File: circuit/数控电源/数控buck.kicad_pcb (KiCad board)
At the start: 2 copper layers, 50 x 50 mm, 80 parts, among them J1 Conn_01x06_MountingPin, J2 Conn_01x02, J5 Conn_01x02, Q1 BSC070N10NS3G, Q2 BSC070N10NS3G, SW1 SW_Push, U1 STM32F334R8Tx, U2 LM5164DDA, U4 LM5109MA, U5 INA240A1PW, U6 TLV9062, U8 LM2675M-5, Y1 Crystal_GND24

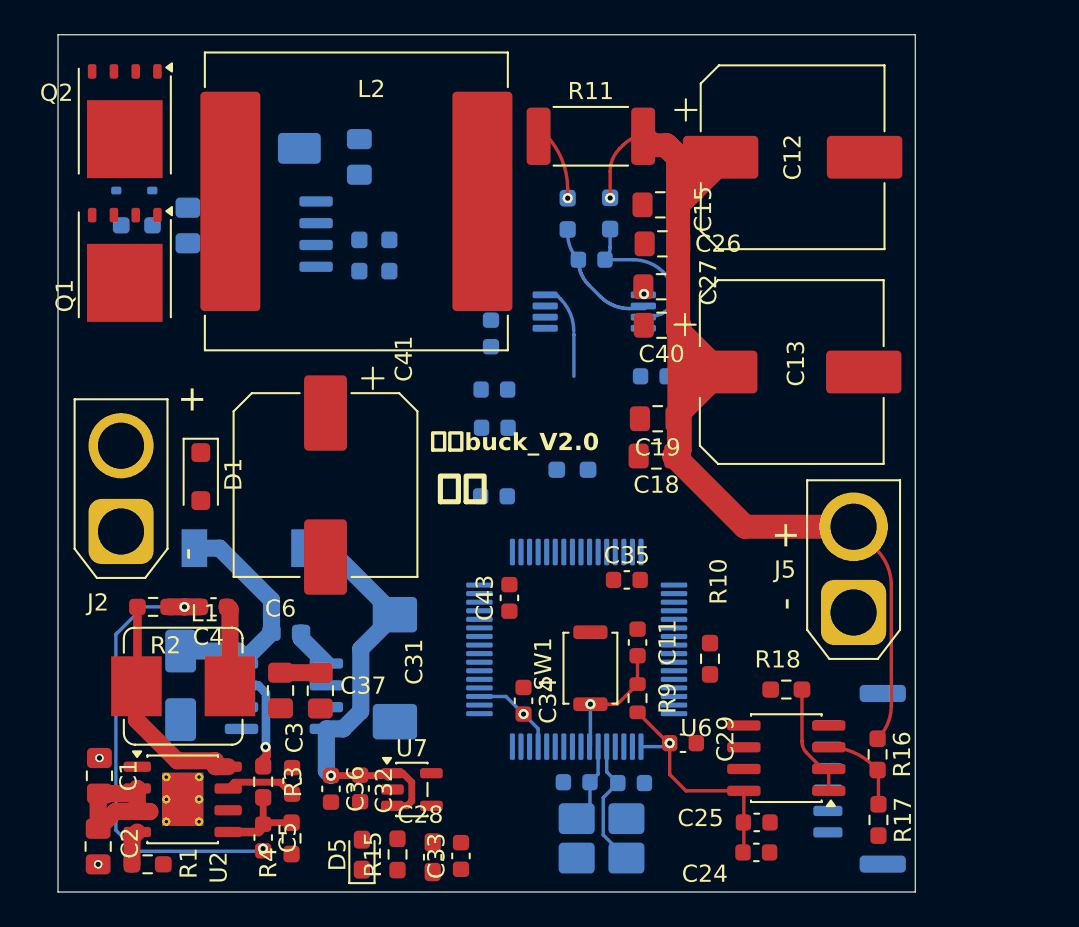
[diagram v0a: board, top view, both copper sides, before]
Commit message: 完成第二版电路版布局
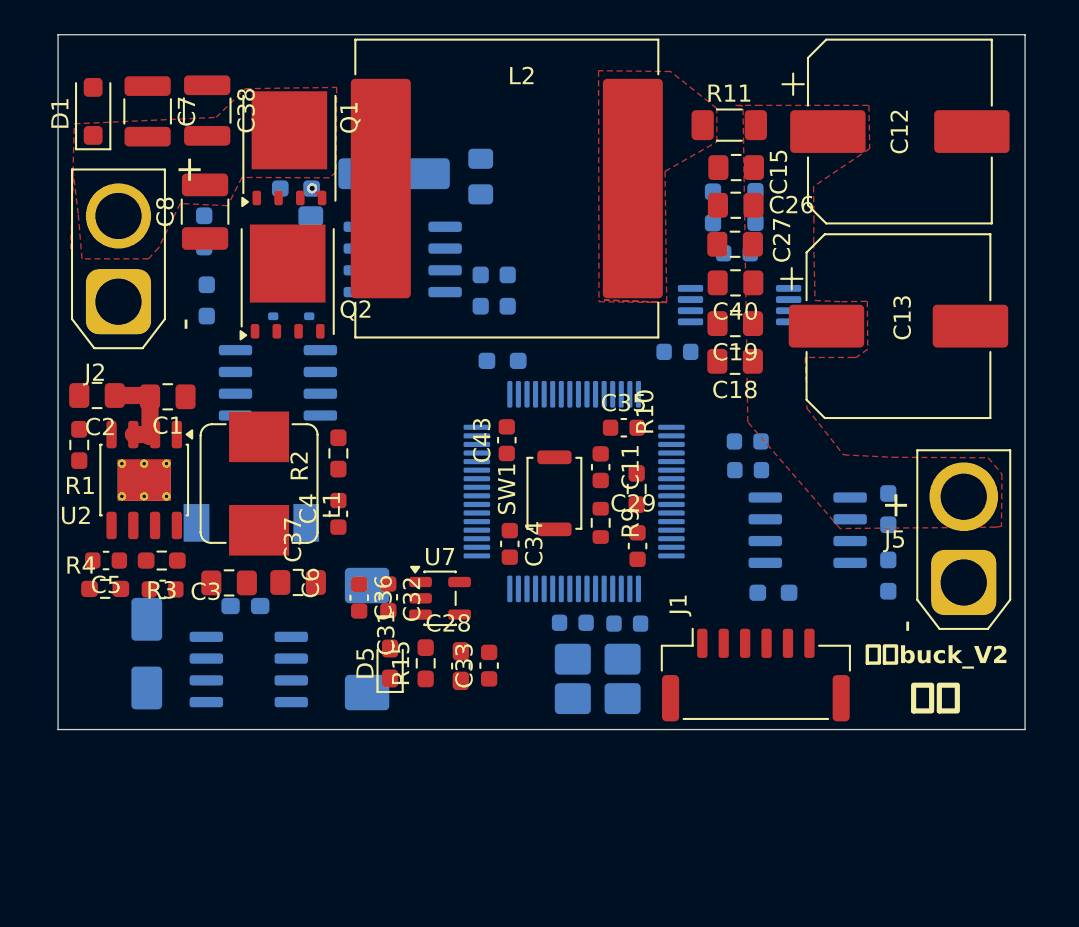
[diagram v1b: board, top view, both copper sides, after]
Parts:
- removed C17, C20: 100n, Capacitor_SMD:C_0603_1608Metric
- removed C23, C39: 2.2u, Capacitor_SMD:C_0603_1608Metric
- removed C41: 100u, Capacitor_SMD:CP_Elec_10x10.5
- added C38: 10u, Capacitor_SMD:C_1210_3225Metric, F.Cu at (23.4, 43.2)
- added C7: 10u, Capacitor_SMD:C_1210_3225Metric, F.Cu at (20.0, 43.3)
- added C8: 10u, Capacitor_SMD:C_1210_3225Metric_Pad1.33x2.70mm_HandSolder, F.Cu at (23.3, 49.1)
- added R19: 27k, Resistor_SMD:R_0603_1608Metric_Pad0.98x0.95mm_HandSolder, B.Cu at (23.3, 50.3)
- added R20: 3k, Resistor_SMD:R_0603_1608Metric_Pad0.98x0.95mm_HandSolder, B.Cu at (23.4, 54.3)
- added U3: TLV9062, Package_SO:SOIC-8_3.9x4.9mm_P1.27mm, B.Cu at (27.6, 59.1)
- C24, C25, R16, R17, R18, U6: moved to B.Cu
- J1: moved to F.Cu
- R11: footprint Resistor_SMD:R_2512_6332Metric_Pad1.40x3.35mm_HandSolder -> Resistor_SMD:R_1206_3216Metric_Pad1.30x1.75mm_HandSolder
- moved C2 26.3 mm to (17.0, 59.9), turned to 180 degrees
- moved R1 24.8 mm to (16.0, 62.8), turned to -90 degrees
- moved C1 22.5 mm to (21.1, 59.9), turned to 0 degrees
- moved C24 22.3 mm to (55.0, 64.2), turned to 0 degrees
- moved C25 22.2 mm to (55.0, 62.5), turned to 0 degrees
- moved D1 22.2 mm to (16.8, 43.3), turned to 90 degrees
- moved U2 18.8 mm to (19.8, 64.8), turned to -90 degrees
- moved C5 18.6 mm to (17.6, 69.5), turned to 180 degrees
- moved R4 18.2 mm to (17.5, 71.2), turned to 0 degrees
- moved R16 14.3 mm to (63.2, 66.5)
- moved R17 14.3 mm to (63.2, 70.4)
- moved R3 14.2 mm to (20.8, 69.5), turned to 0 degrees
- moved R2 14.0 mm to (31.1, 63.2), turned to -90 degrees
- moved C3 13.5 mm to (20.9, 71.2), turned to 0 degrees
- moved J2 13.4 mm to (18.3, 54.4)
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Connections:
- U1 pad 35: unconnected-(U1-PB14-Pad35) -> /adc_Vin
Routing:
- net +24V: track 67.2 -> 0.00 mm, vias 1 -> 0
- net Net-(C4-Pad1): track 27.1 -> 0.00 mm, vias 2 -> 0
- net +5V: track 26.0 -> 0.00 mm, vias 1 -> 0
- net +3.3V: track 19.8 -> 0.00 mm, vias 2 -> 0
- net Net-(D13-K): track 13.6 -> 0.00 mm
- net Net-(U2-SW): track 13.3 -> 0.00 mm
- net +12V: track 13.2 -> 0.00 mm, vias 1 -> 0
- net Net-(U5--): track 9.00 -> 0.00 mm
- net /OSC_IN: track 7.68 -> 0.00 mm
- net Net-(U5-+): track 7.56 -> 0.00 mm
- net /NRST: track 7.38 -> 0.00 mm, vias 1 -> 0
- net /comp_volt: track 7.32 -> 0.00 mm
- net Net-(U2-FB): track 5.77 -> 0.00 mm
- net /comp_cirurt: track 5.53 -> 0.00 mm
- net Net-(U6A-+): track 5.24 -> 0.00 mm
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- added copper zone on F.Cu, net +24V
- added copper zone on F.Cu, net +48V
- added copper zone on F.Cu, net Net-(L2-Pad2)
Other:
- board size 50 x 50 mm -> 56.4 x 40.5 mm
- board text added: "数控buck_V2"
- board text removed: "数控buck_V2.0"
